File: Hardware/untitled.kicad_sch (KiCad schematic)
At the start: 16 parts, among them IC1 LM74502HDDFR, J3 CarLVPowerConnector, Q2 PSMN8R5-40MSDX

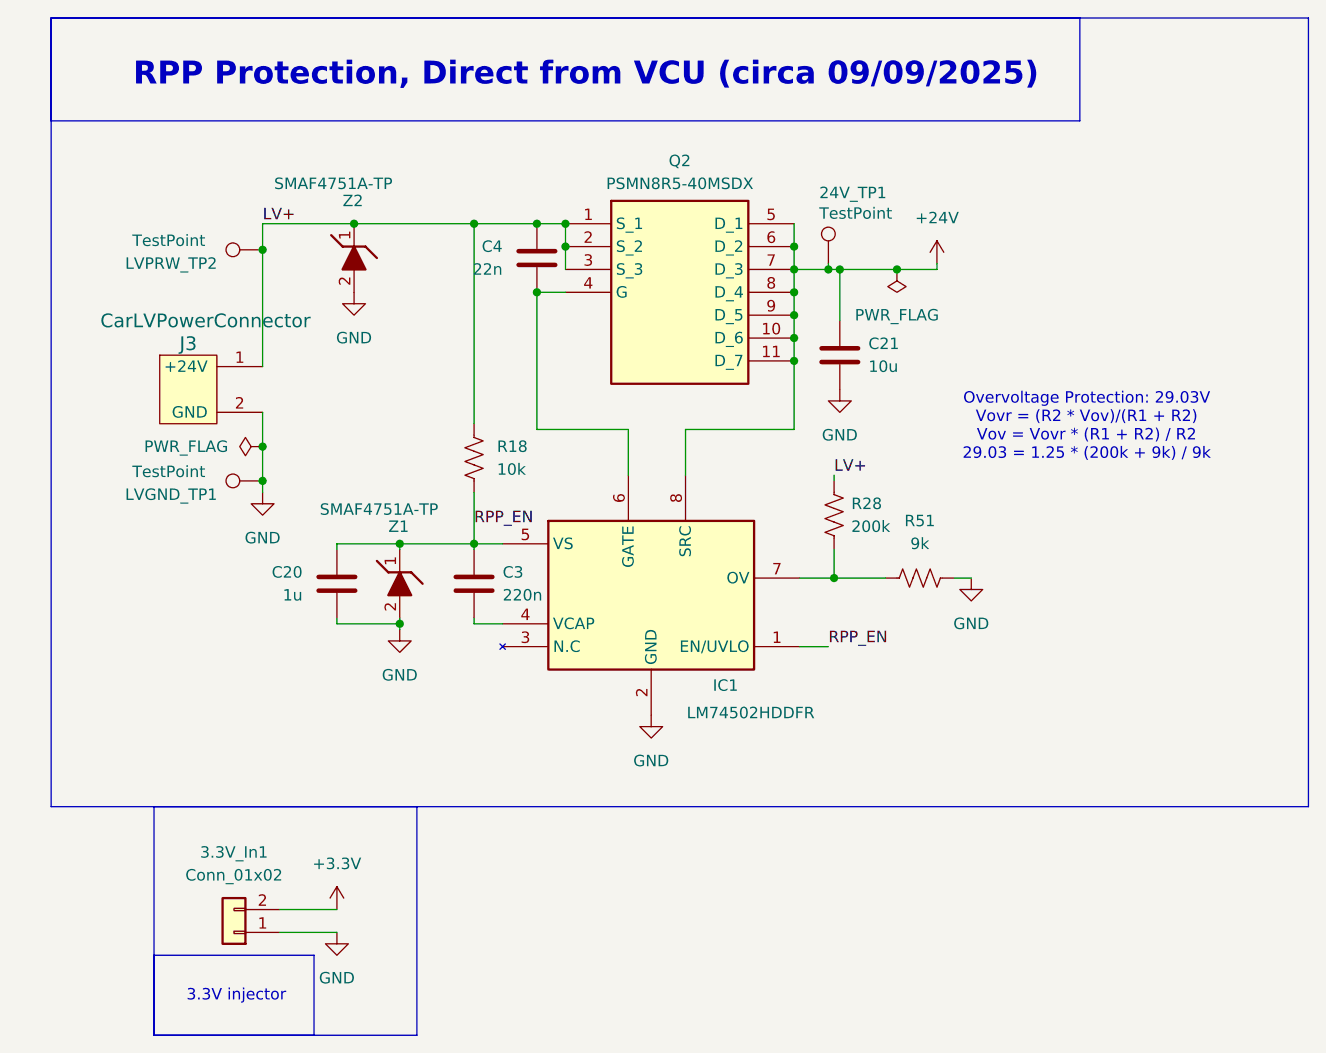
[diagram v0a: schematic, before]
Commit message: Backup
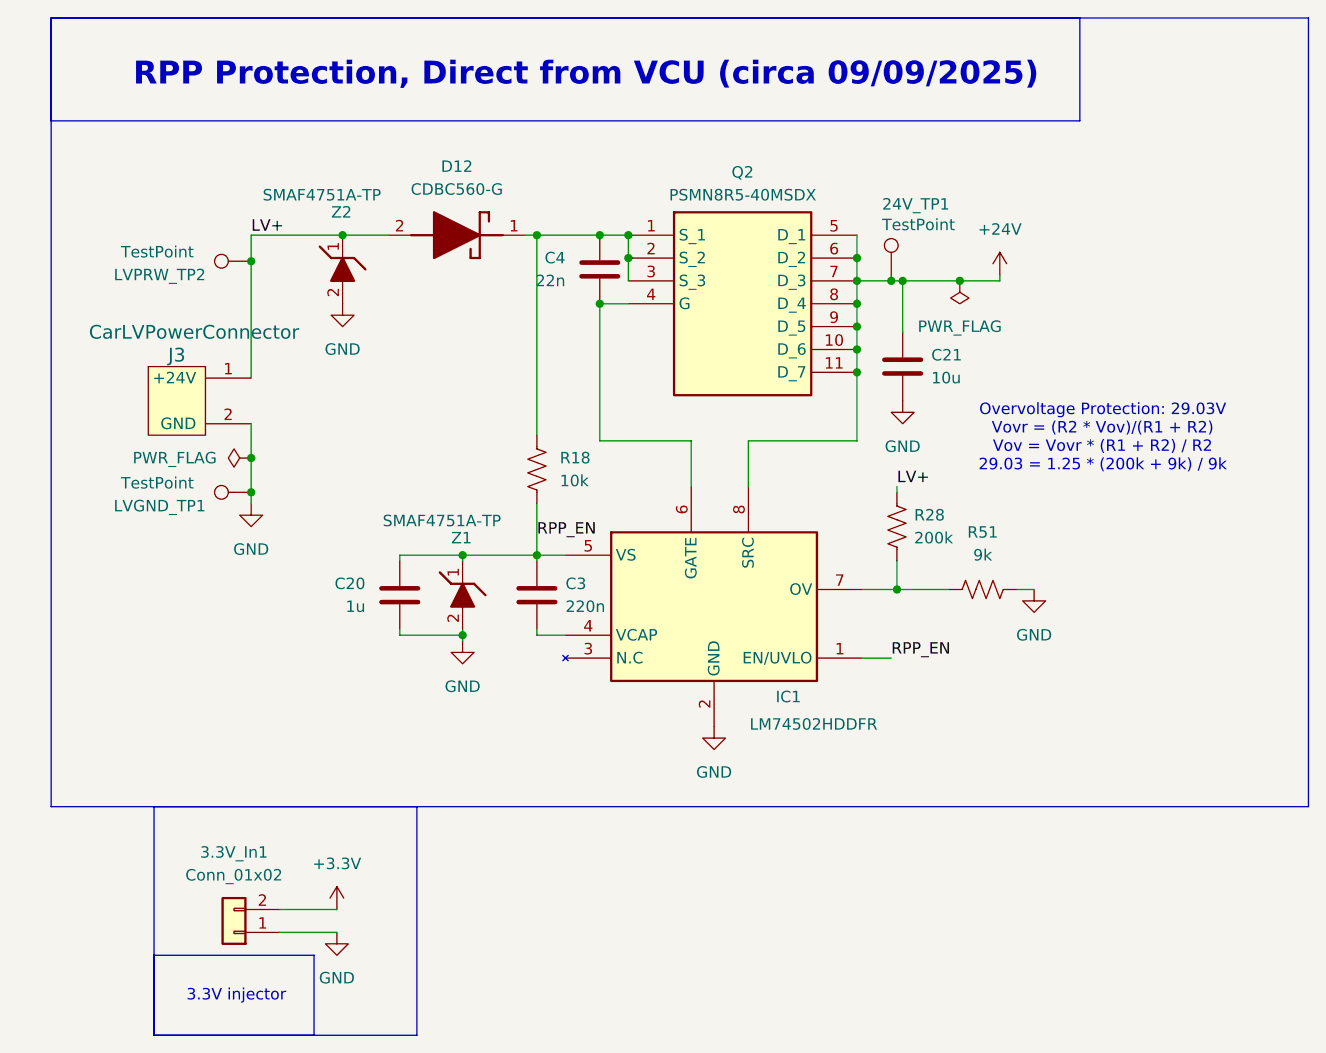
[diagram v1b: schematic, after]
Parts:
- added D12: CDBC560-G, Schlotty:DIOM7959X262N, symbol Schott:CDBC560-G
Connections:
- net LV+: now also D12.2 (A); no longer C4.2, Q2.1 (S_1), Q2.2 (S_2), Q2.3 (S_3), R18.1
- new net: C4.2, D12.1 (K), Q2.1 (S_1), Q2.2 (S_2), Q2.3 (S_3), R18.1
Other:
- moved on the sheet: 24V_TP1, C20, C21, C3, C4, IC1, J3, LVGND_TP1, LVPRW_TP2, Q2, R18, R28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
